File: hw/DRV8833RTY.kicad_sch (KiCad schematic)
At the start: 9 parts, among them U7 DRV8833RTY

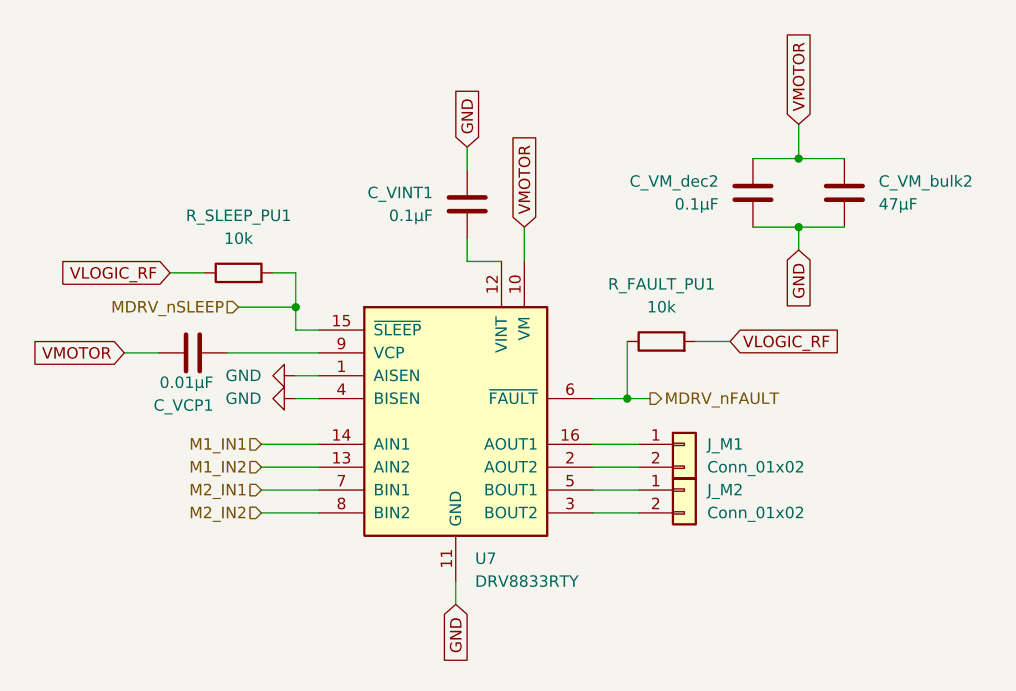
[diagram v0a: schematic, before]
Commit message: WIP
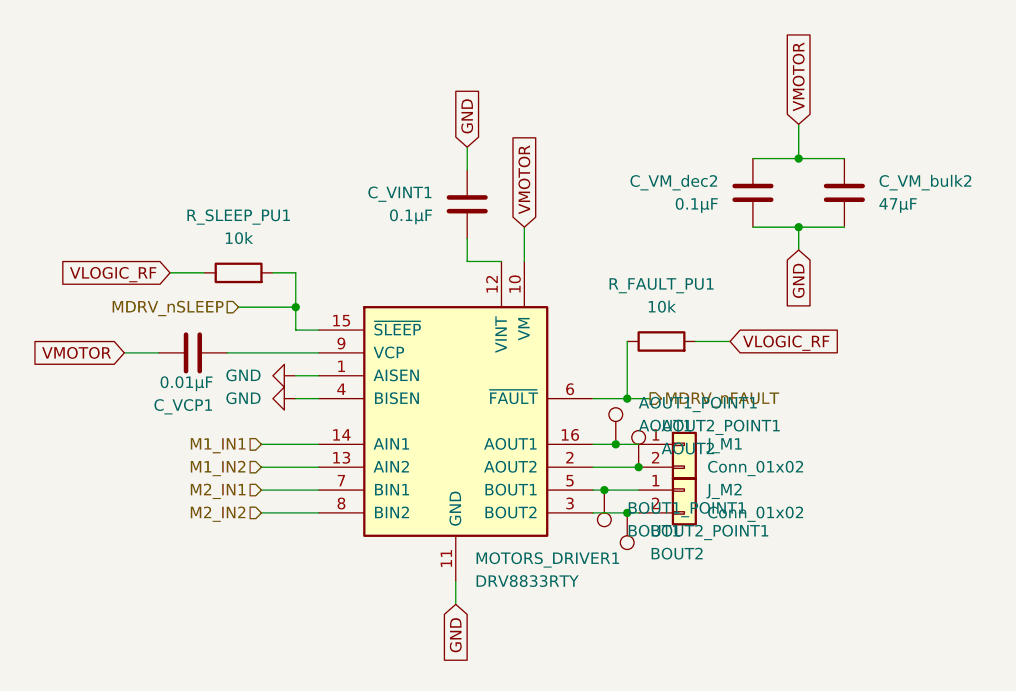
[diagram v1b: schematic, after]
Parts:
- added AOUT1_POINT1: AOUT1, TestPoint:TestPoint_Pad_1.0x1.0mm, symbol Connector:TestPoint
- added AOUT2_POINT1: AOUT2, TestPoint:TestPoint_Pad_1.0x1.0mm, symbol Connector:TestPoint
- added BOUT1_POINT1: BOUT1, TestPoint:TestPoint_Pad_1.0x1.0mm, symbol Connector:TestPoint
- added BOUT2_POINT1: BOUT2, TestPoint:TestPoint_Pad_1.0x1.0mm, symbol Connector:TestPoint
- renumbered U7 to MOTORS_DRIVER1
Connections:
- net at J_M1.1 (Pin_1), MOTORS_DRIVER1.16 (AOUT1): now also AOUT1_POINT1.1
- net at J_M1.2 (Pin_2), MOTORS_DRIVER1.2 (AOUT2): now also AOUT2_POINT1.1
- net at J_M2.2 (Pin_2), MOTORS_DRIVER1.3 (BOUT2): now also BOUT2_POINT1.1
- net at J_M2.1 (Pin_1), MOTORS_DRIVER1.5 (BOUT1): now also BOUT1_POINT1.1
